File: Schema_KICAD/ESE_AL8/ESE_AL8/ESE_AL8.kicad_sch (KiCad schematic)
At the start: 23 parts, among them J101 ECRAN, J102 GPIO, U101 STM32G431CBUx, Y101 16MHz

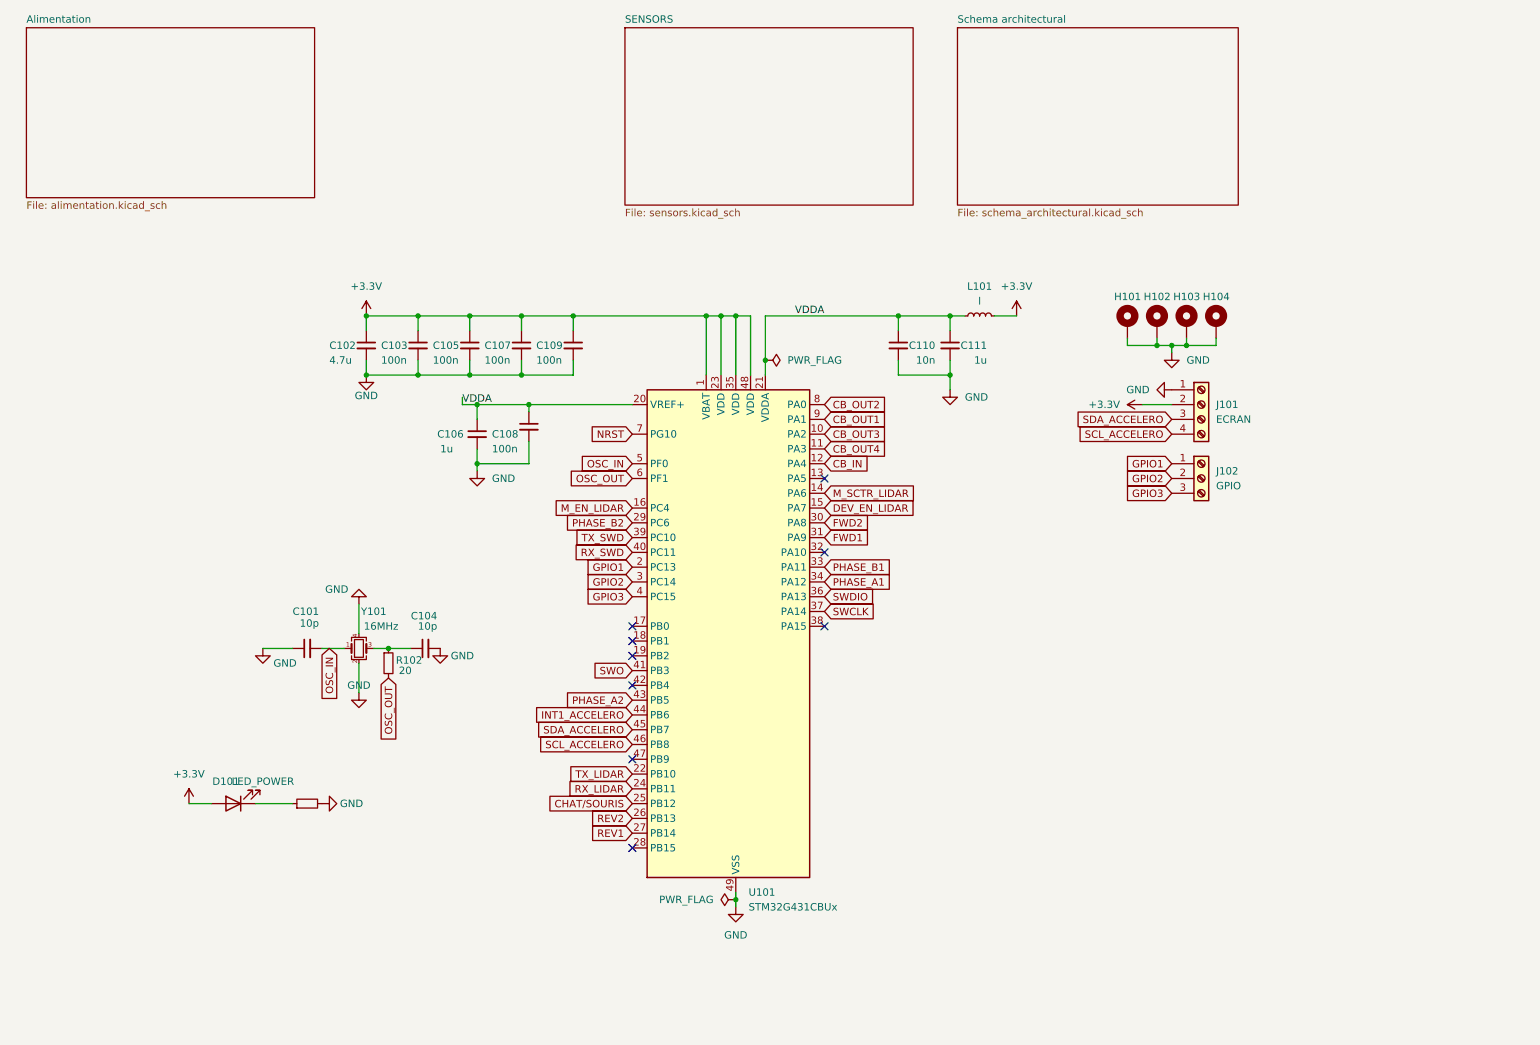
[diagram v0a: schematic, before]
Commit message: commit AL08_1
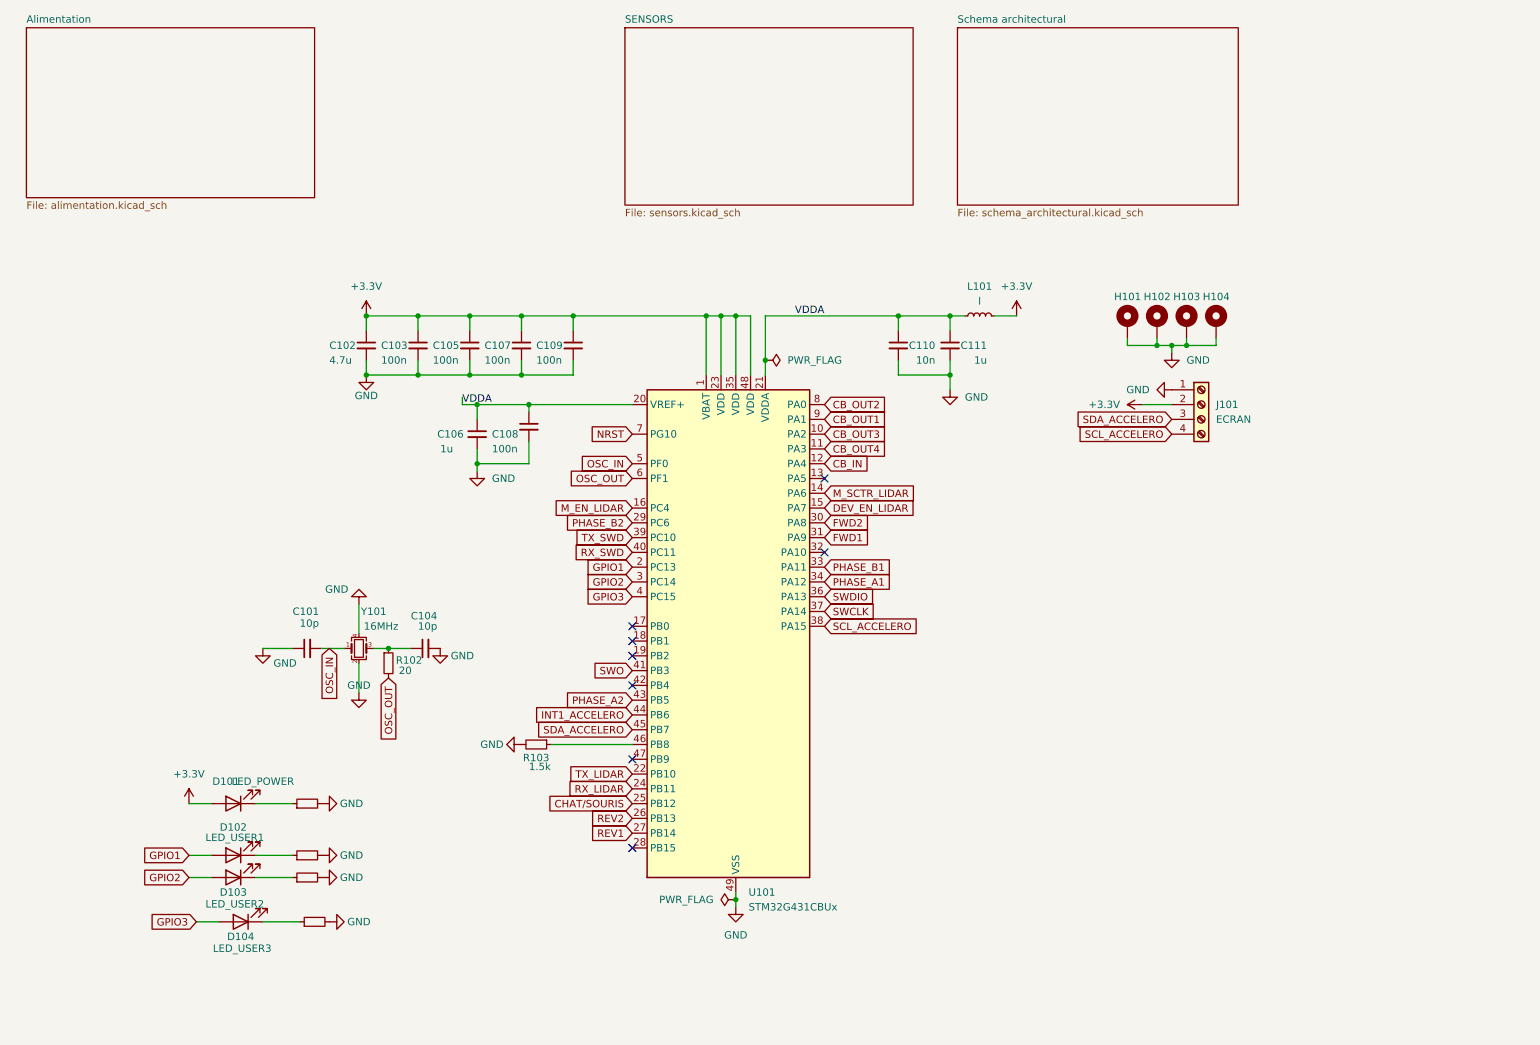
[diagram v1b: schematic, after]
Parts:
- removed J102: GPIO, Connector_PinSocket_2.54mm:PinSocket_1x03_P2.54mm_Vertical, symbol Connector:Screw_Terminal_01x03
- added D102: LED_USER1, Resistor_SMD:R_0402_1005Metric_Pad0.72x0.64mm_HandSolder, symbol Device:LED
- added D103: LED_USER2, Resistor_SMD:R_0402_1005Metric_Pad0.72x0.64mm_HandSolder, symbol Device:LED
- added D104: LED_USER3, Resistor_SMD:R_0402_1005Metric_Pad0.72x0.64mm_HandSolder, symbol Device:LED
- added R103: 1.5k, Resistor_SMD:R_0402_1005Metric_Pad0.72x0.64mm_HandSolder, symbol Device:R_Small
- added R104, R105, R106: 680, Resistor_SMD:R_0402_1005Metric_Pad0.72x0.64mm_HandSolder, symbol Device:R_Small
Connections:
- net GND: now also R103.2, R104.2, R105.2, R106.2
- net GPIO1: now also D102.2 (A)
- net GPIO2: now also D103.2 (A)
- net GPIO3: now also D104.2 (A)
- net SCL_ACCELERO: now also U101.38 (PA15); no longer U101.46 (PB8)
- new net: R103.1, U101.46 (PB8)
- new net: D104.1 (K), R106.1
- new net: D103.1 (K), R105.1
- new net: D102.1 (K), R104.1
- no-connect marks 9 -> 8

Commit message: commit du code et kicad modifié
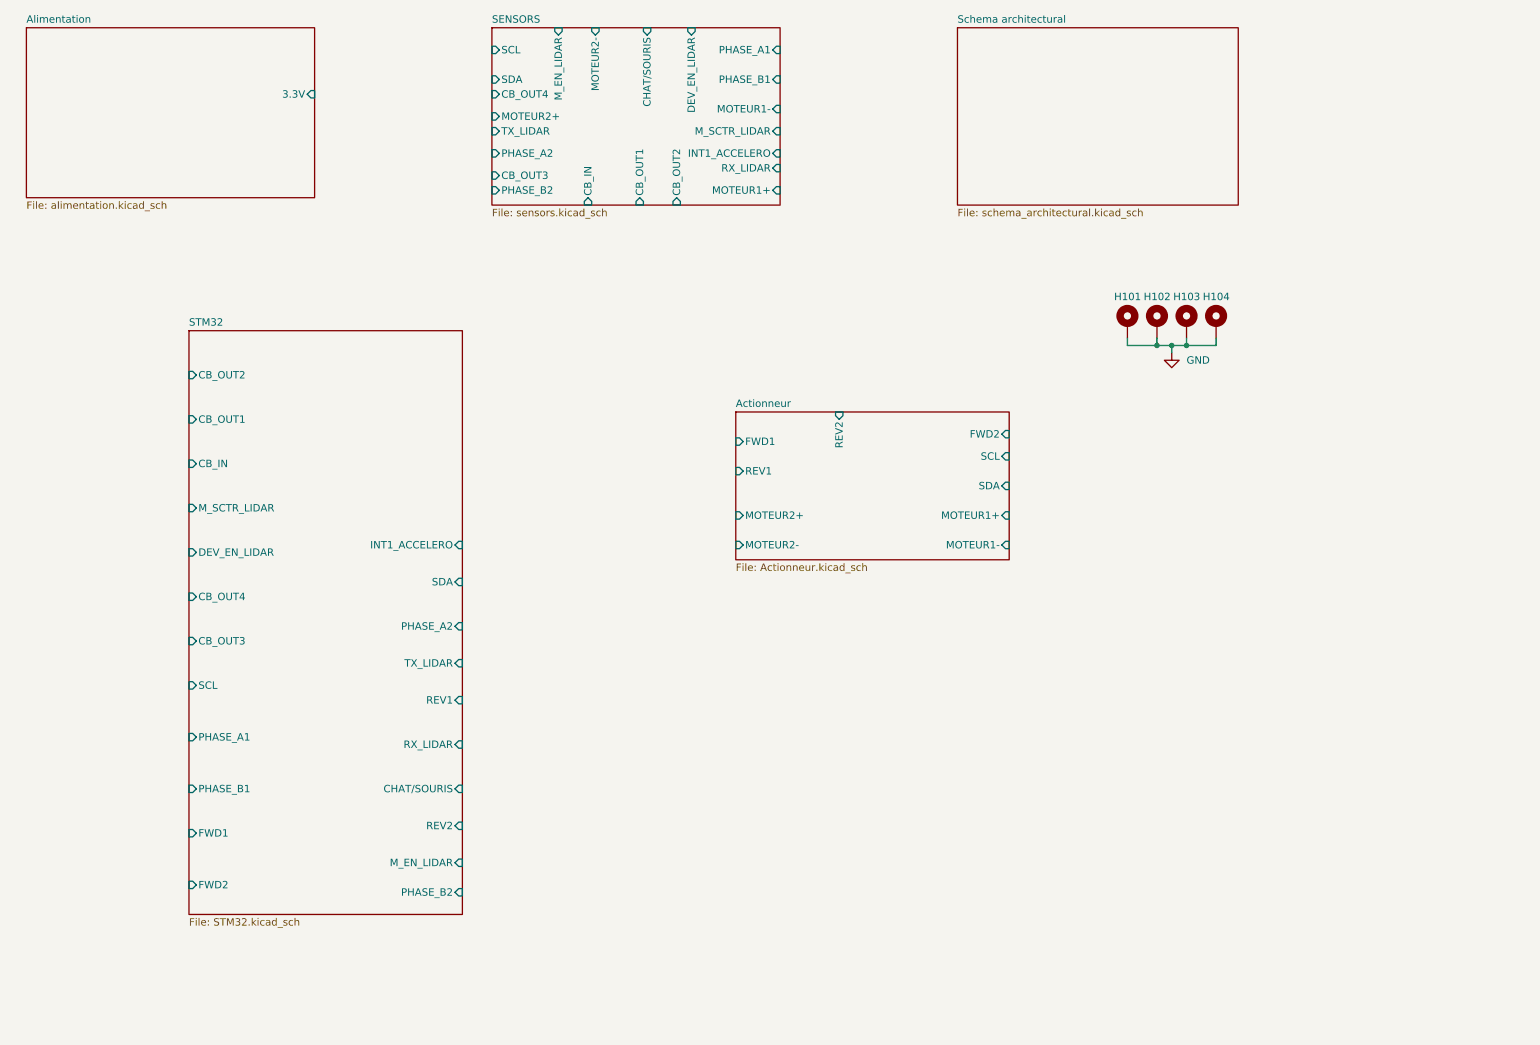
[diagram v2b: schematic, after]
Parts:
- removed C101, C104: 10p, Capacitor_SMD:C_0402_1005Metric_Pad0.74x0.62mm_HandSolder, symbol Device:C_Small
- removed C102: 4.7u, Capacitor_SMD:C_0603_1608Metric_Pad1.08x0.95mm_HandSolder, symbol Device:C_Small
- removed C103, C105, C107, C108, C109: 100n, Capacitor_SMD:C_0402_1005Metric_Pad0.74x0.62mm_HandSolder, symbol Device:C_Small
- removed C106, C111: 1u, Capacitor_SMD:C_0402_1005Metric_Pad0.74x0.62mm_HandSolder, symbol Device:C_Small
- removed C110: 10n, Capacitor_SMD:C_0402_1005Metric_Pad0.74x0.62mm_HandSolder, symbol Device:C_Small
- removed D101: LED_POWER, Resistor_SMD:R_0402_1005Metric_Pad0.72x0.64mm_HandSolder, symbol Device:LED
- removed D102: LED_USER1, Resistor_SMD:R_0402_1005Metric_Pad0.72x0.64mm_HandSolder, symbol Device:LED
- removed D103: LED_USER2, Resistor_SMD:R_0402_1005Metric_Pad0.72x0.64mm_HandSolder, symbol Device:LED
- removed D104: LED_USER3, Resistor_SMD:R_0402_1005Metric_Pad0.72x0.64mm_HandSolder, symbol Device:LED
- removed J101: ECRAN, Connector_PinSocket_2.54mm:PinSocket_1x04_P2.54mm_Vertical, symbol Connector:Screw_Terminal_01x04
- removed L101: l, Capacitor_SMD:C_0402_1005Metric_Pad0.74x0.62mm_HandSolder, symbol Device:L_Small
- removed R101, R104, R105, R106: 680, Resistor_SMD:R_0402_1005Metric_Pad0.72x0.64mm_HandSolder, symbol Device:R_Small
- removed R102: 20, Resistor_SMD:R_0402_1005Metric_Pad0.72x0.64mm_HandSolder, symbol Device:R_Small
- removed R103: 1.5k, Resistor_SMD:R_0402_1005Metric_Pad0.72x0.64mm_HandSolder, symbol Device:R_Small
- removed U101: STM32G431CBUx, STM32:QFN-48-1EP_7x7mm_P0.5mm_EP5.6x5.6mm_AJ, symbol MCU_ST_STM32G4:STM32G431CBUx
- removed Y101: 16MHz, Crystal:Crystal_SMD_3225-4Pin_3.2x2.5mm, symbol Device:Crystal_GND24_Small
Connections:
- no-connect marks 8 -> 0
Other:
- added sheet Actionneur (Actionneur.kicad_sch)
- added sheet STM32 (STM32.kicad_sch)
- sheet Alimentation ports: added 3.3V; removed none
- sheet SENSORS ports: added CB_IN, CB_OUT1, CB_OUT2, CB_OUT3, CB_OUT4, CHAT/SOURIS, DEV_EN_LIDAR, INT1_ACCELERO, MOTEUR1+, MOTEUR1-, MOTEUR2+, MOTEUR2-, M_EN_LIDAR, M_SCTR_LIDAR, PHASE_A1, PHASE_A2, PHASE_B1, PHASE_B2, RX_LIDAR, SCL, SDA, TX_LIDAR; removed none

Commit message: commit pour le schema
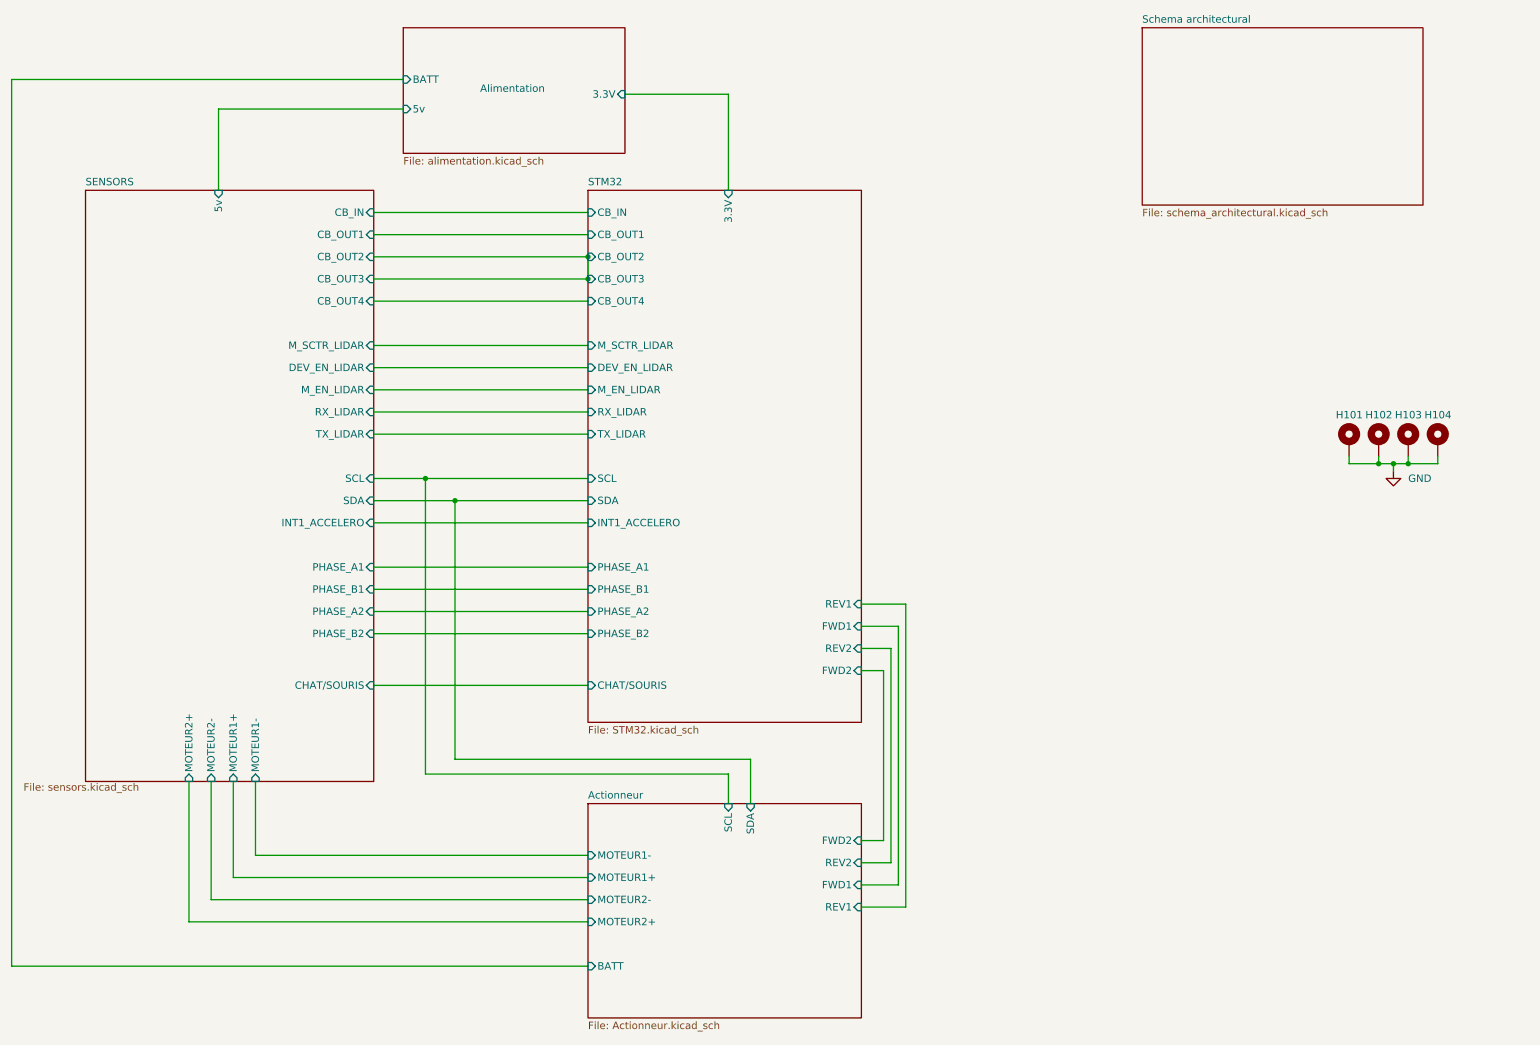
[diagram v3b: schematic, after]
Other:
- sheet Actionneur ports: added BATT; removed none
- sheet Alimentation ports: added 5v, BATT; removed none
- sheet SENSORS ports: added 5v; removed none
- sheet STM32 ports: added 3.3V; removed none
- moved on the sheet: H101, H102, H103, H104
